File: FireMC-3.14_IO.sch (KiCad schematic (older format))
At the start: 2 parts

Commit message: math check
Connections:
- net labels removed: +5F
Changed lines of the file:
@@
 $EndComp
 $Comp
-L +5F #PWR025
-U 1 1 57CB7400
+L +5V #PWR026
+U 1 1 57CB7418
 P 4950 900
-F 0 "#PWR025" H 4950 750 50  0001 C CNN
-F 1 "+5F" H 4950 1040 50  0000 C CNN
+F 0 "#PWR026" H 4950 750 50  0001 C CNN
+F 1 "+5V" H 4950 1040 50  0000 C CNN
 F 2 "" H 4950 900 50  0000 C CNN
 F 3 "" H 4950 900 50  0000 C CNN
@@
 	1    0    0    -1
 $EndComp
-$Comp
-L +5V #PWR026
-U 1 1 57CB7418
-P 3850 900
-F 0 "#PWR026" H 3850 750 50  0001 C CNN
-F 1 "+5V" H 3850 1040 50  0000 C CNN
-F 2 "" H 3850 900 50  0000 C CNN
-F 3 "" H 3850 900 50  0000 C CNN
-	1    3850 900
-	1    0    0    -1
-$EndComp

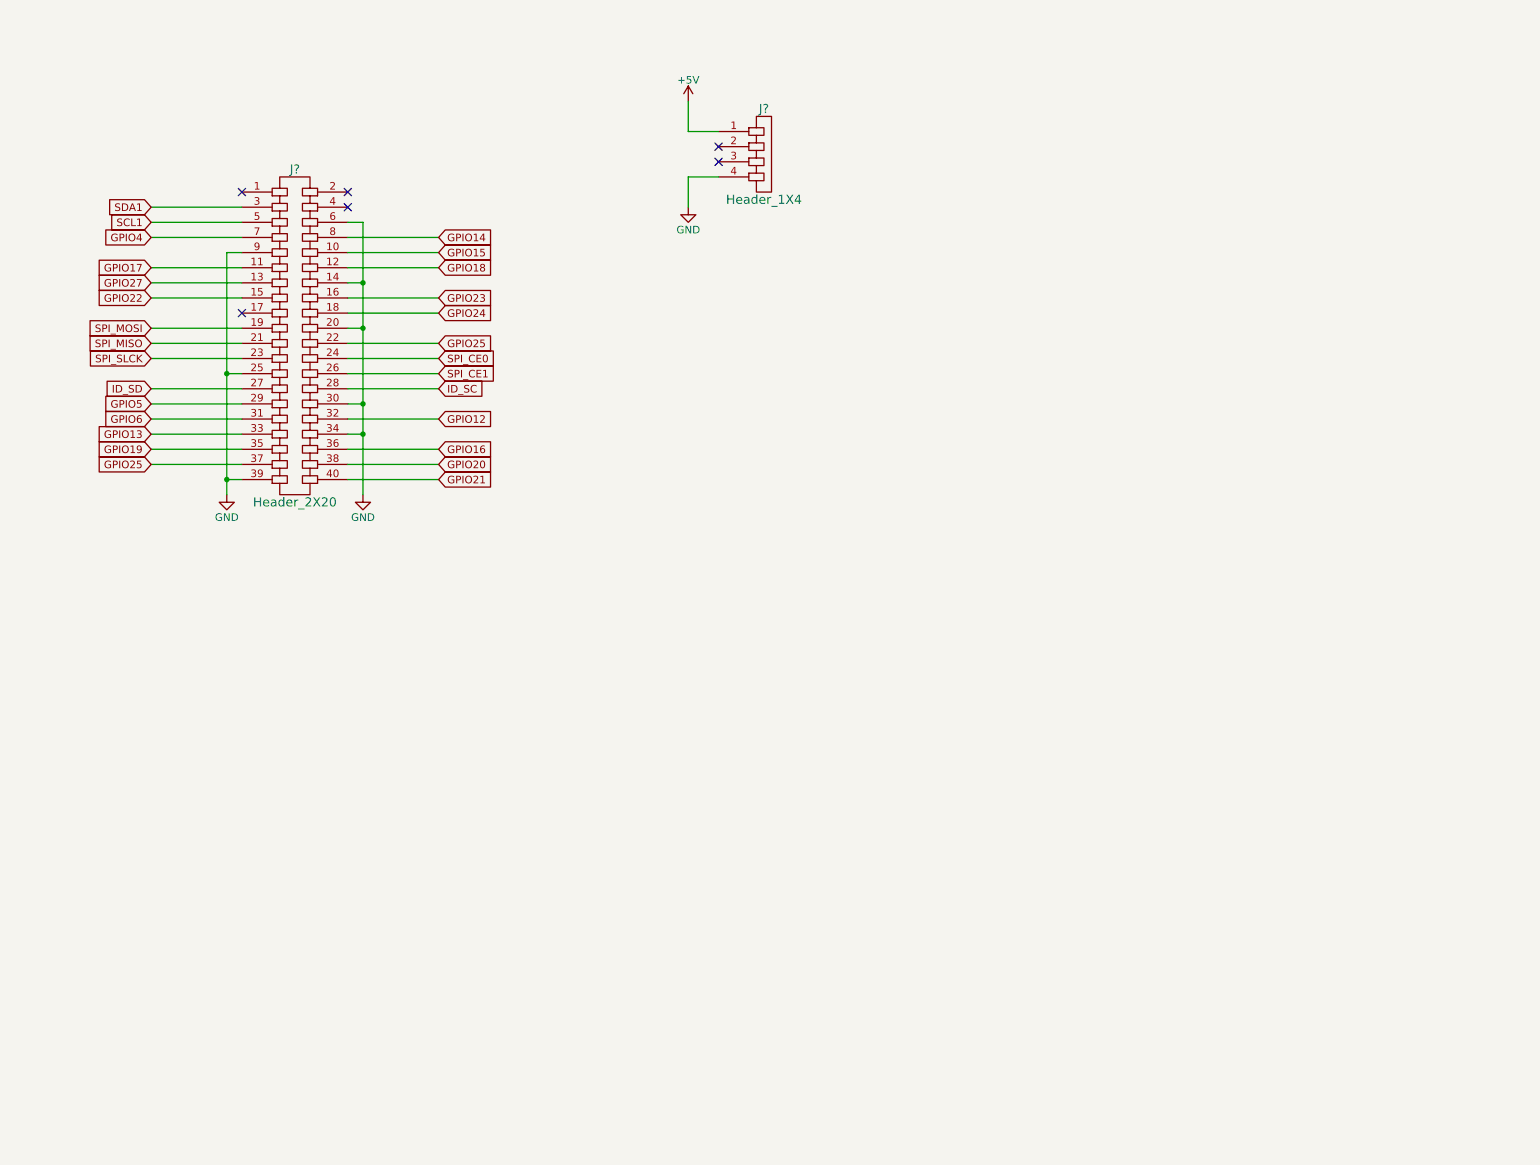
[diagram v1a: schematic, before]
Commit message: Schematic 80% complete
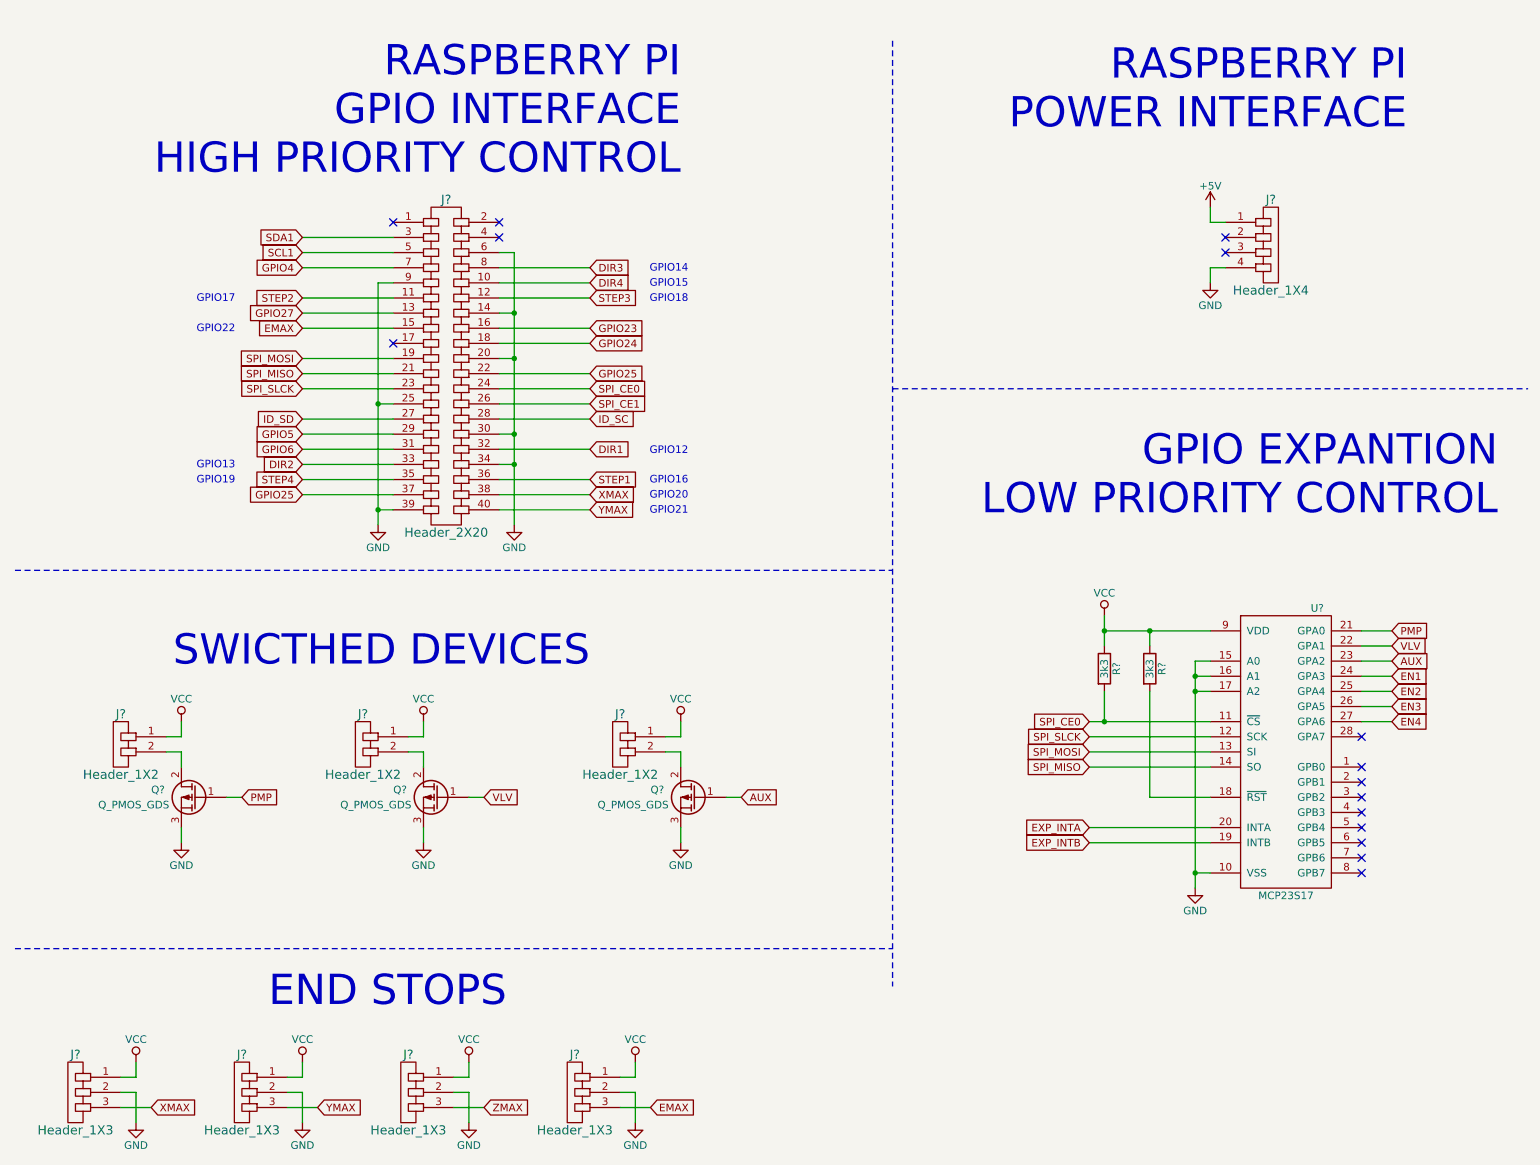
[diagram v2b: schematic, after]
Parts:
- added J? (x3): Header_1X2, symbol Header_1X2
- added J? (x4): Header_1X3, symbol Header_1X3
- added Q? (x3): Q_PMOS_GDS, symbol Q_PMOS_GDS
- added R? (x2): 3k3, symbol R
- added U?: MCP23S17, symbol MCP23S17
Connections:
- net GND: now also J?.2, J?.2, J?.2, J?.2, Q?.3 (S), Q?.3 (S), Q?.3 (S), U?.10 (VSS), U?.15 (A0), U?.16 (A1), U?.17 (A2)
- net SPI_CE0: now also R?.2, U?.11 (~CS)
- net SPI_MISO: now also U?.14 (SO)
- net SPI_MOSI: now also U?.13 (SI)
- net SPI_SLCK: now also U?.12 (SCK)
- net GPIO12 renamed DIR1
- net GPIO13 renamed DIR2
- net GPIO14 renamed DIR3
- net GPIO15 renamed DIR4
- net GPIO16 renamed STEP1
- net GPIO17 renamed STEP2
- net GPIO18 renamed STEP3
- net GPIO19 renamed STEP4
- net GPIO20 renamed XMAX
- net XMAX: now also J?.3
- net GPIO21 renamed YMAX
- net YMAX: now also J?.3
- net GPIO22 renamed EMAX
- net EMAX: now also J?.3
- new net: J?.2, Q?.2 (D) (x3)
- new net: R?.2, U?.18 (~RST)
- new net AUX: Q?.1 (G), U?.23 (GPA2)
- new net EN1: U?.24 (GPA3)
- new net EN2: U?.25 (GPA4)
- new net EN3: U?.26 (GPA5)
- new net EN4: U?.27 (GPA6)
- new net EXP_INTA: U?.20 (INTA)
- new net EXP_INTB: U?.19 (INTB)
- new net PMP: Q?.1 (G), U?.21 (GPA0)
- new net VCC: J?.1, J?.1, J?.1, J?.1, J?.1, J?.1, J?.1, R?.1, R?.1, U?.9 (VDD)
- new net VLV: Q?.1 (G), U?.22 (GPA1)
- new net ZMAX: J?.3
- no-connect marks 6 -> 15
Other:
- note added: "END STOPS"
- note added: "GPIO EXPANTION\nLOW PRIORITY CONTROL"
- note added: "GPIO12"
- note added: "GPIO13"
- note added: "GPIO14"
- note added: "GPIO15"
- note added: "GPIO16"
- note added: "GPIO17"
- note added: "GPIO18"
- note added: "GPIO19"
- note added: "GPIO20"
- note added: "GPIO21"
- note added: "GPIO22"
- note added: "RASPBERRY PI\nGPIO INTERFACE\nHIGH PRIORITY CONTROL"
- note added: "RASPBERRY PI\nPOWER INTERFACE"
- note added: "SWICTHED DEVICES"
- moved on the sheet: J?
